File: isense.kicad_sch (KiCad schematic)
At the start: 8 parts, among them U1 TLV2372

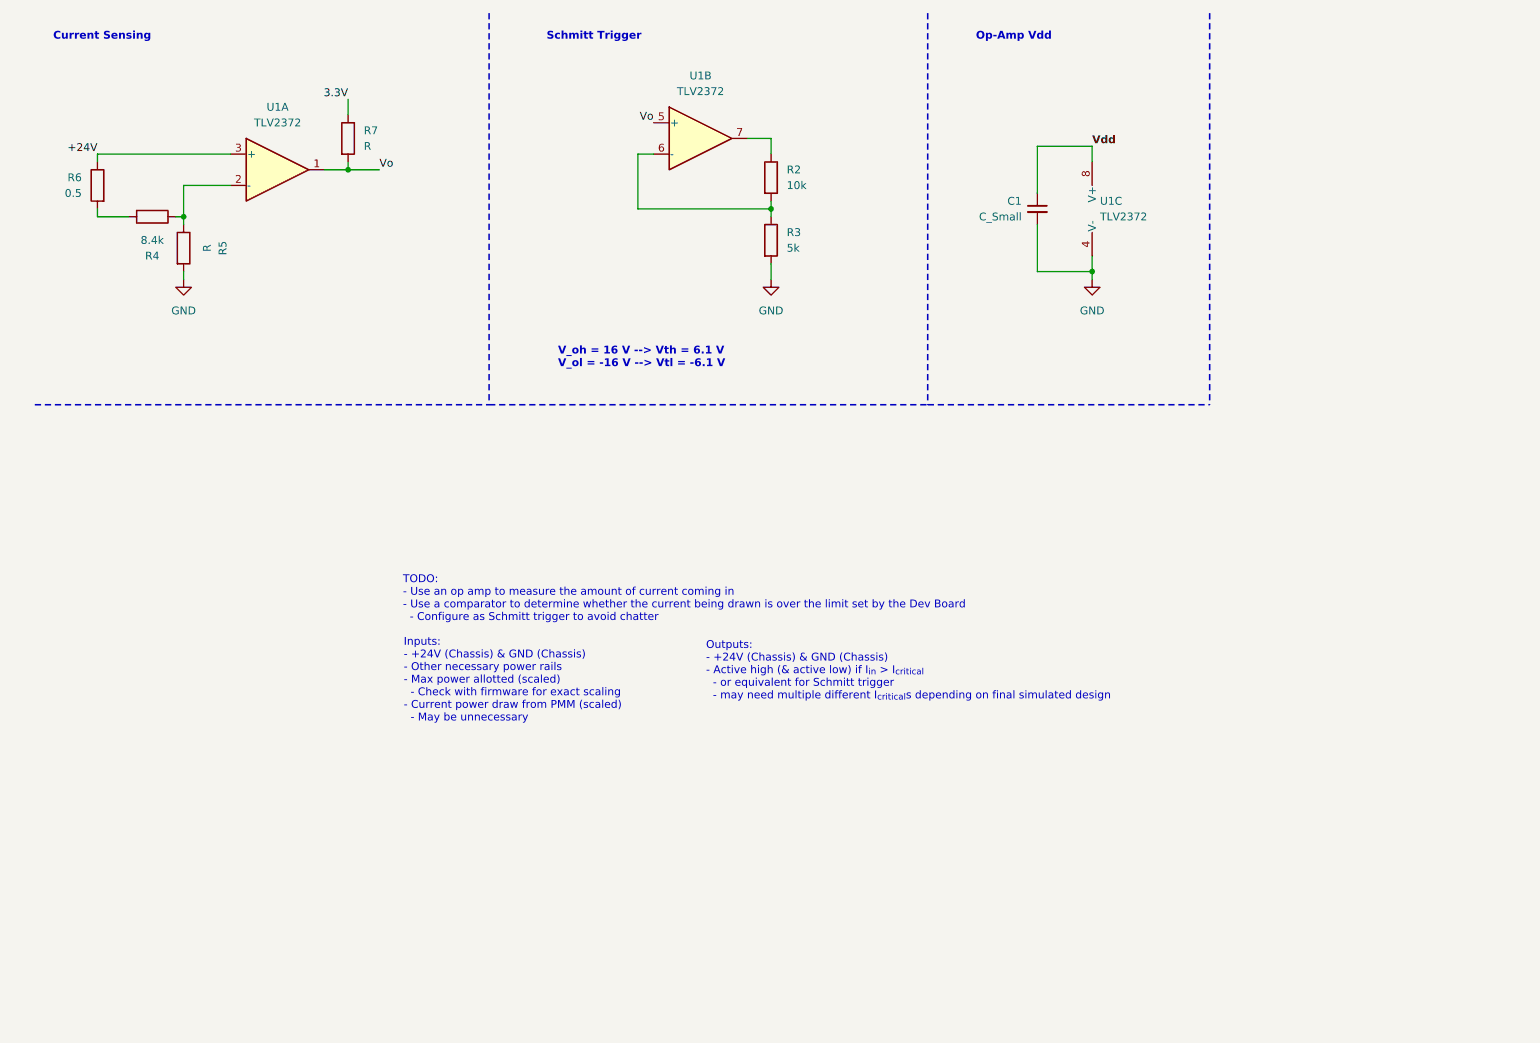
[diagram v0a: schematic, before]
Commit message: Trying to do current sense but it's not fun
canercanercnarennc
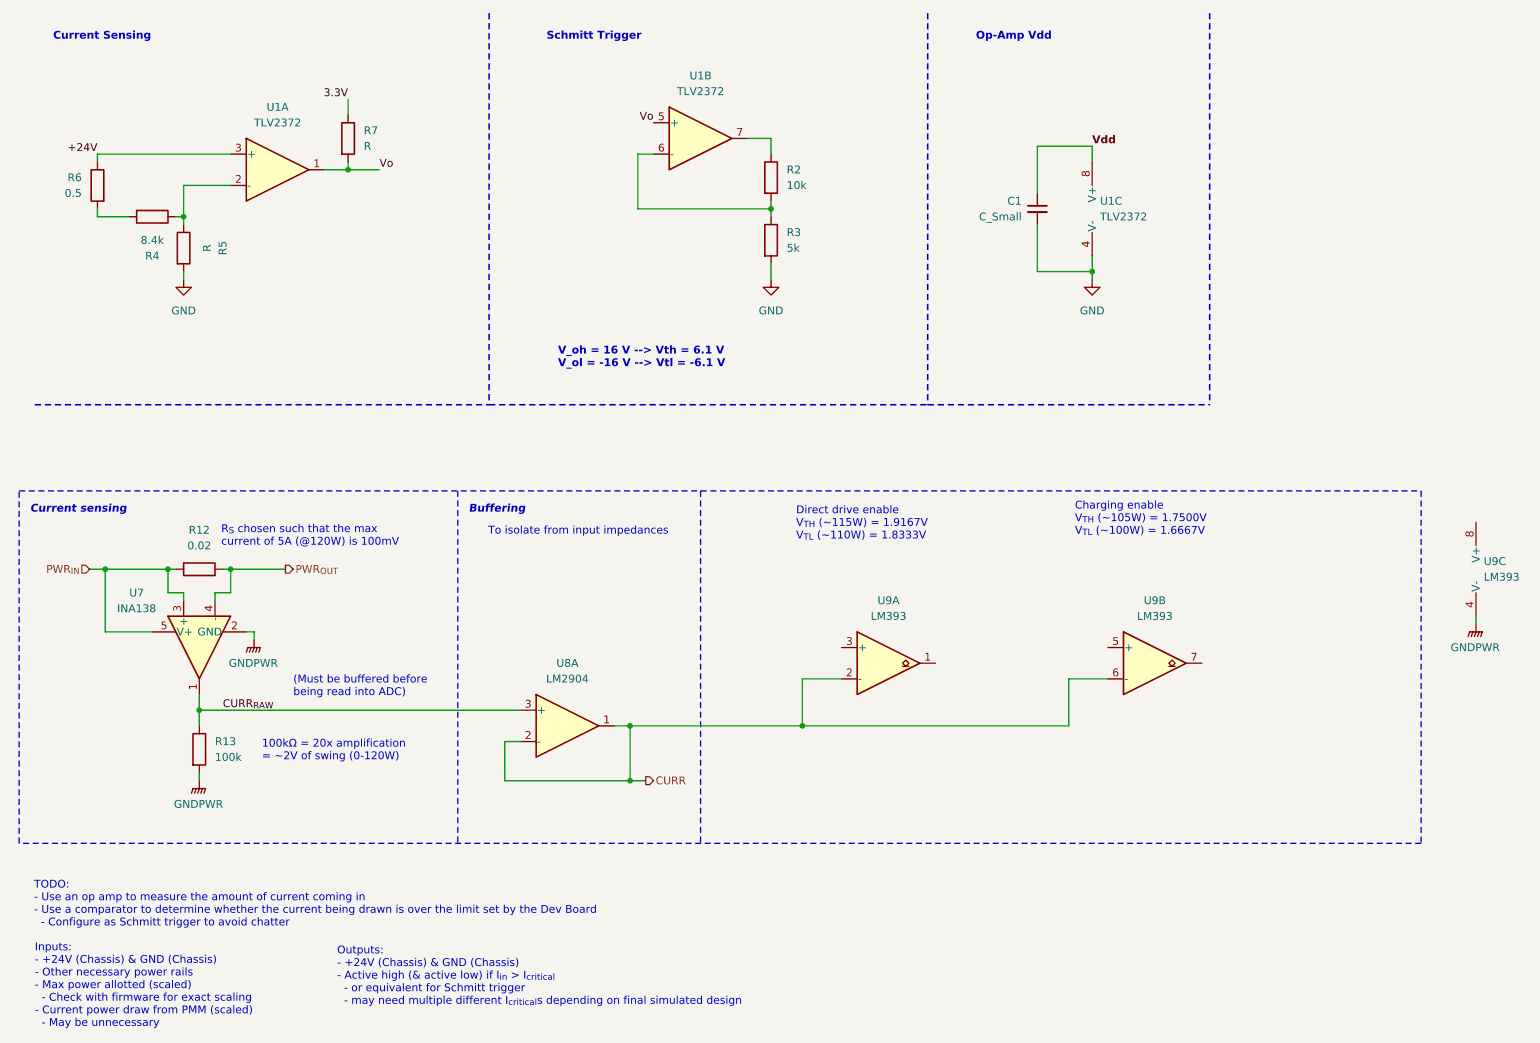
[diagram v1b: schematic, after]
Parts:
- added R12: 0.02, Resistor_SMD:R_0805_2012Metric_Pad1.20x1.40mm_HandSolder, symbol Device:R
- added R13: 100k, Resistor_SMD:R_0603_1608Metric_Pad0.98x0.95mm_HandSolder, symbol Device:R
- added U7: INA138, Package_TO_SOT_SMD:SOT-23_Handsoldering, symbol Amplifier_Current:INA138
- added U8: LM2904, Package_SO:SOIC-8_3.9x4.9mm_P1.27mm, symbol Amplifier_Operational:LM2904
- added U9: LM393, Package_SO:SOIC-8_3.9x4.9mm_P1.27mm, symbol Comparator:LM393
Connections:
- new net CURR: U8.1, U8.2 (-), U9.2 (-), U9.6 (-)
- new net CURR_{RAW}: R13.1, U7.1, U8.3 (+)
- new net GNDPWR: R13.2, U7.2 (GND), U9.4 (V-)
- new net PWR_{IN}: R12.1, U7.3 (+), U7.5 (V+)
- new net PWR_{OUT}: R12.2, U7.4 (-)
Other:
- note added: "(Must be buffered before being read into ADC)"
- note added: "100kΩ = 20x amplification = ~2V of swing (0-120W)"
- note added: "Buffering"
- note added: "Charging enable V_{TH} (~105W) = 1.7500V V_{TL} (~100W) = 1.6667V"
- note added: "Current sensing"
- note added: "Direct drive enable V_{TH} (~115W) = 1.9167V V_{TL} (~110W) = 1.8333V"
- note added: "R_{S} chosen such that the max current of 5A (@120W) is 100mV"
- note added: "To isolate from input impedances"
